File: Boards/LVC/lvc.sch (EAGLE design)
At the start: 21 parts, among them Q1 SI7997DP, Q2 RK7002BMT116, U1 NCP300LSN33T1G, U2 L78L33ACUTR, U3 TLV170IDBVR

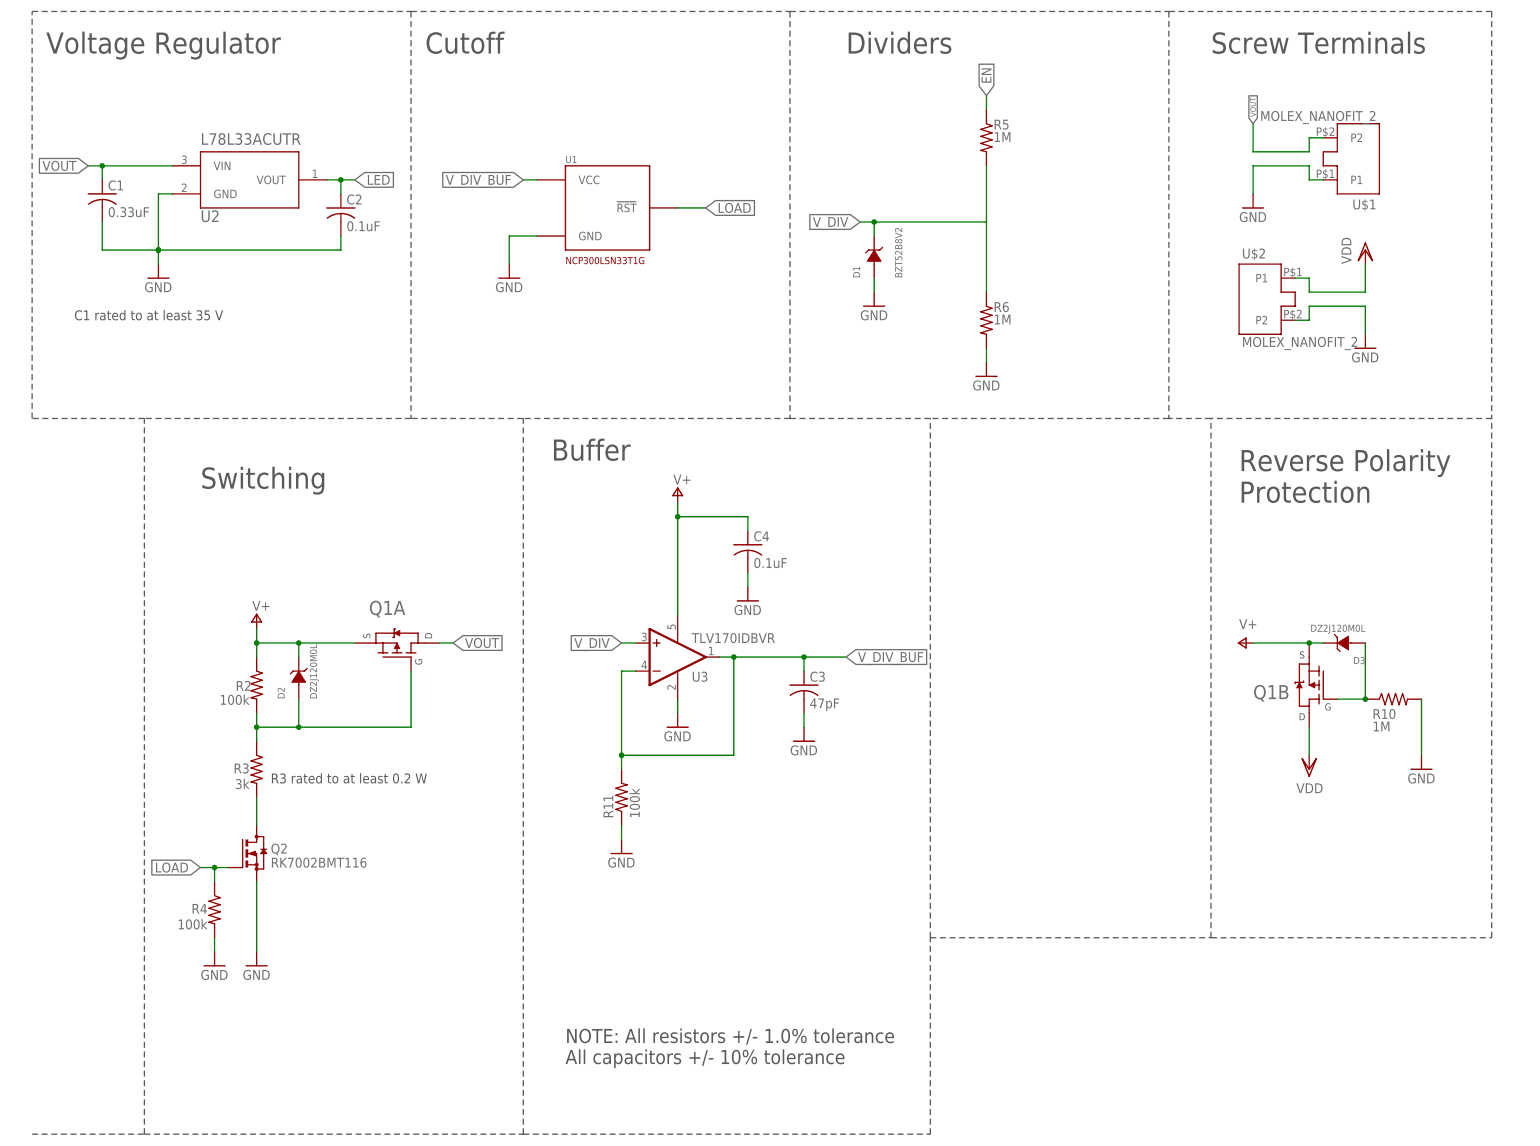
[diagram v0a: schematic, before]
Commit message: All of the changes with CAD and electronics since switching to the microclasp connectors
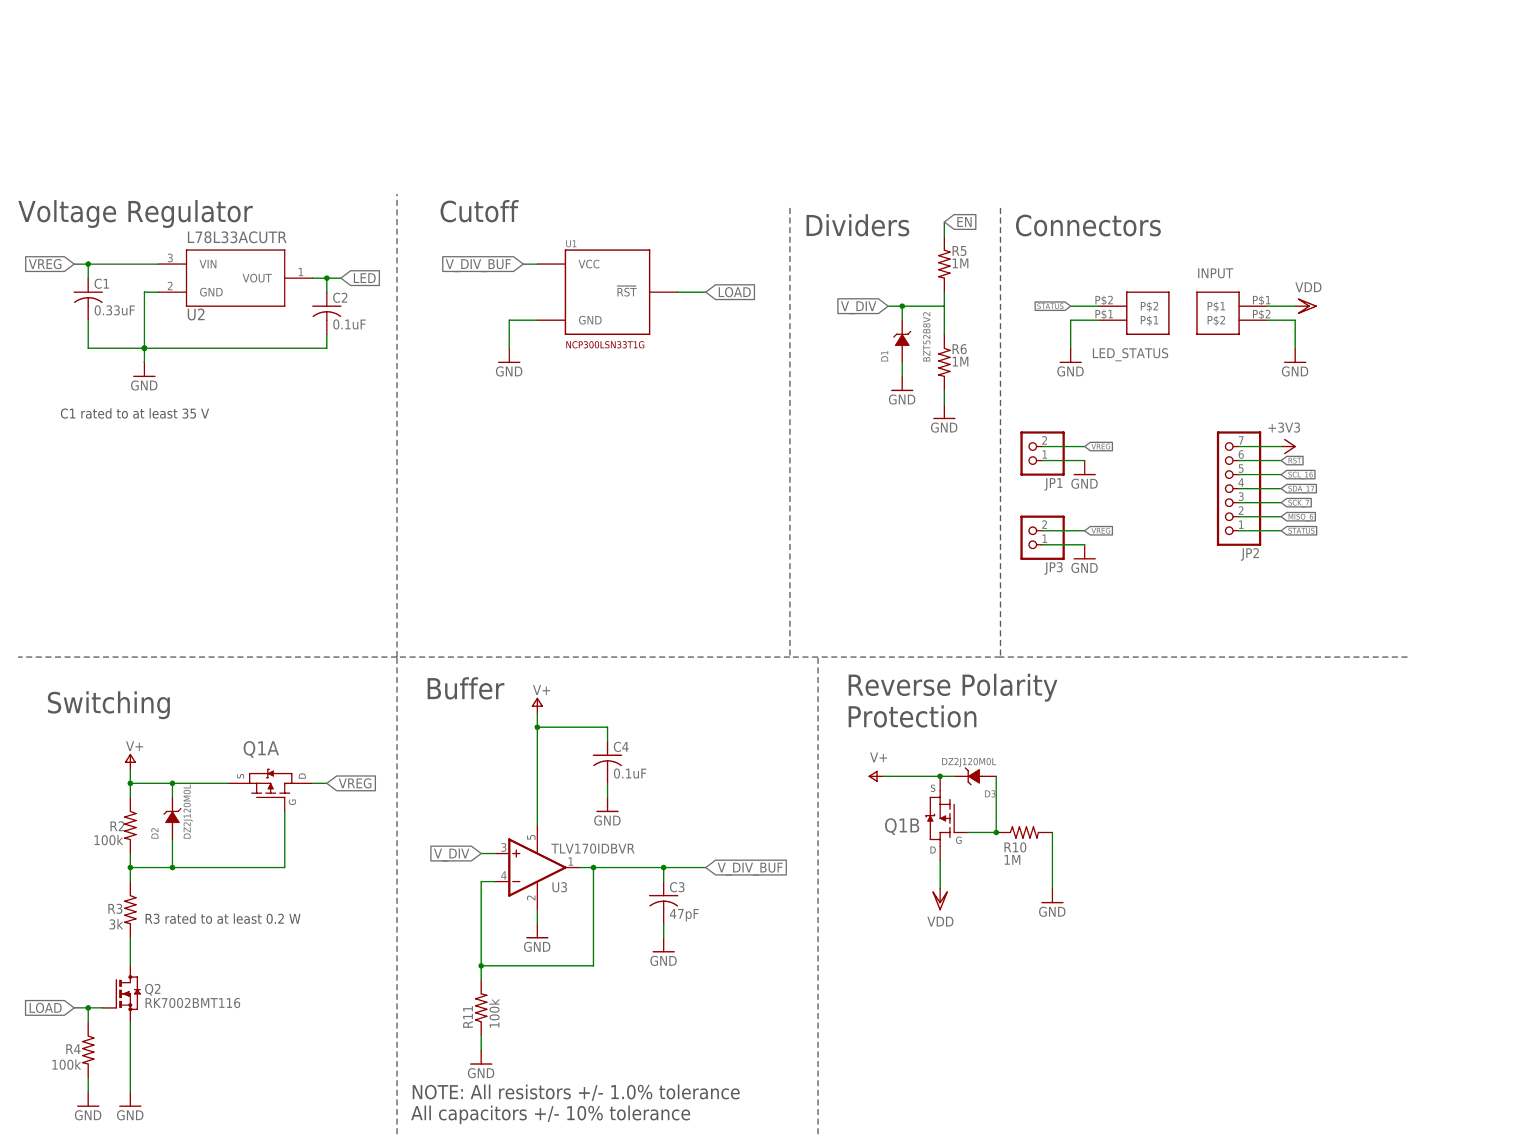
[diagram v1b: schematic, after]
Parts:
- removed U$1, U$2: MOLEX_NANOFIT_2, cmdLibs:MOLEX_NANOFIT_2
- added INPUT, LED_STATUS: (no value), NR_connectors:MICROCLASP
- added JP1, JP3: (no value), pinhead:PINHD-1X2
- added JP2: (no value), pinhead:PINHD-1X7
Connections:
- removed net VOUT: C1.1, Q1A.D, U$1.P2, U2.VIN
- new net MISO_6: JP2.2
- new net N$9: JP2.7
- new net RST: JP2.6
- new net SCK_7: JP2.3
- new net SCL_16: JP2.5
- new net SDA_17: JP2.4
- new net STATUS: JP2.1, LED_STATUS.P$2
- new net VREG: C1.1, JP1.2, JP3.2, Q1A.D, U2.VIN
- net GND: now also INPUT.P$2, JP1.1, JP3.1, LED_STATUS.P$1; no longer U$1.P1, U$2.P2
- net VDD: now also INPUT.P$1; no longer U$2.P1
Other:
- note added: "Connectors"
- note removed: "Screw Terminals"
- moved on the sheet: C1, C2, C3, C4, D1, D2, D3, Q1A, Q1B, Q2, R10, R11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
